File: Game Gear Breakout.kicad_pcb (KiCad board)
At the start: 2 copper layers, 59.1 x 73 mm, 11 parts, among them J1 GG Edge Connector, J2 Logic Analyzer, J3 ROM Chip

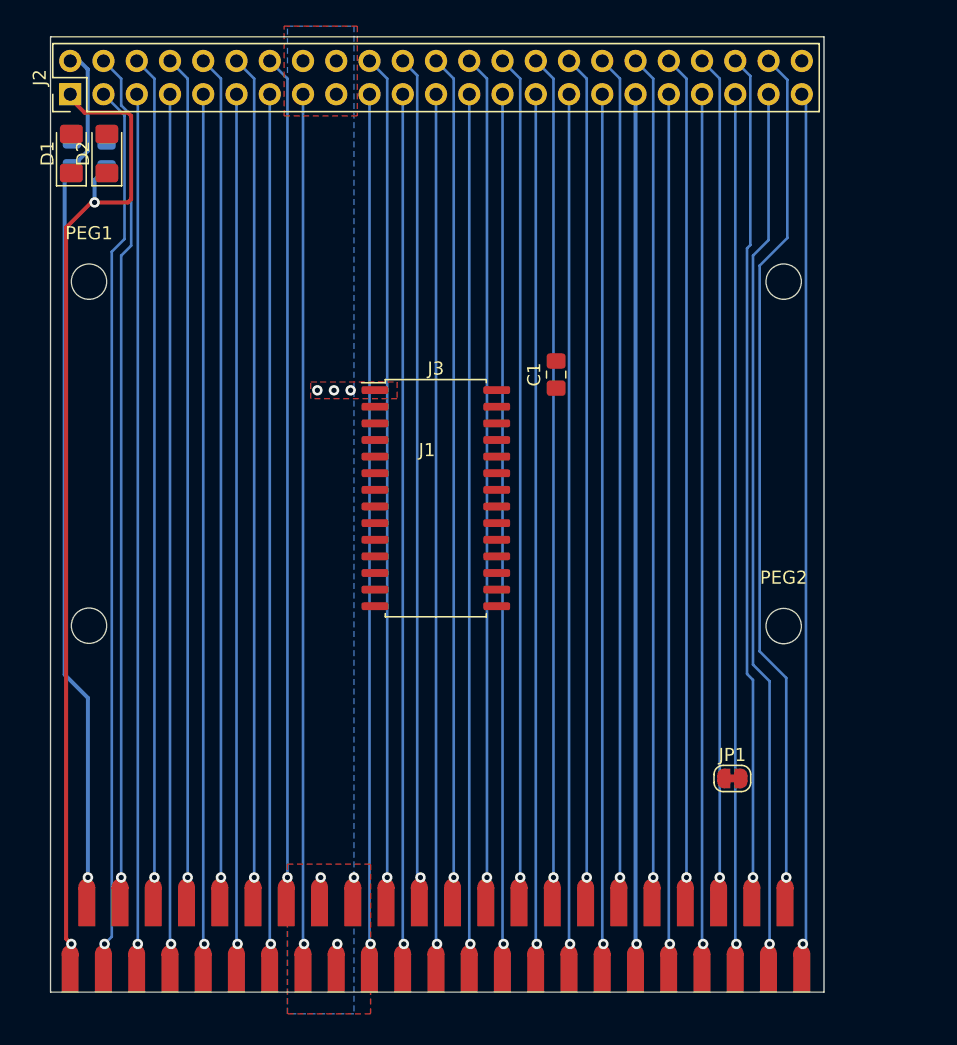
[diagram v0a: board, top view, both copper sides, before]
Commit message: rev1 layout done?
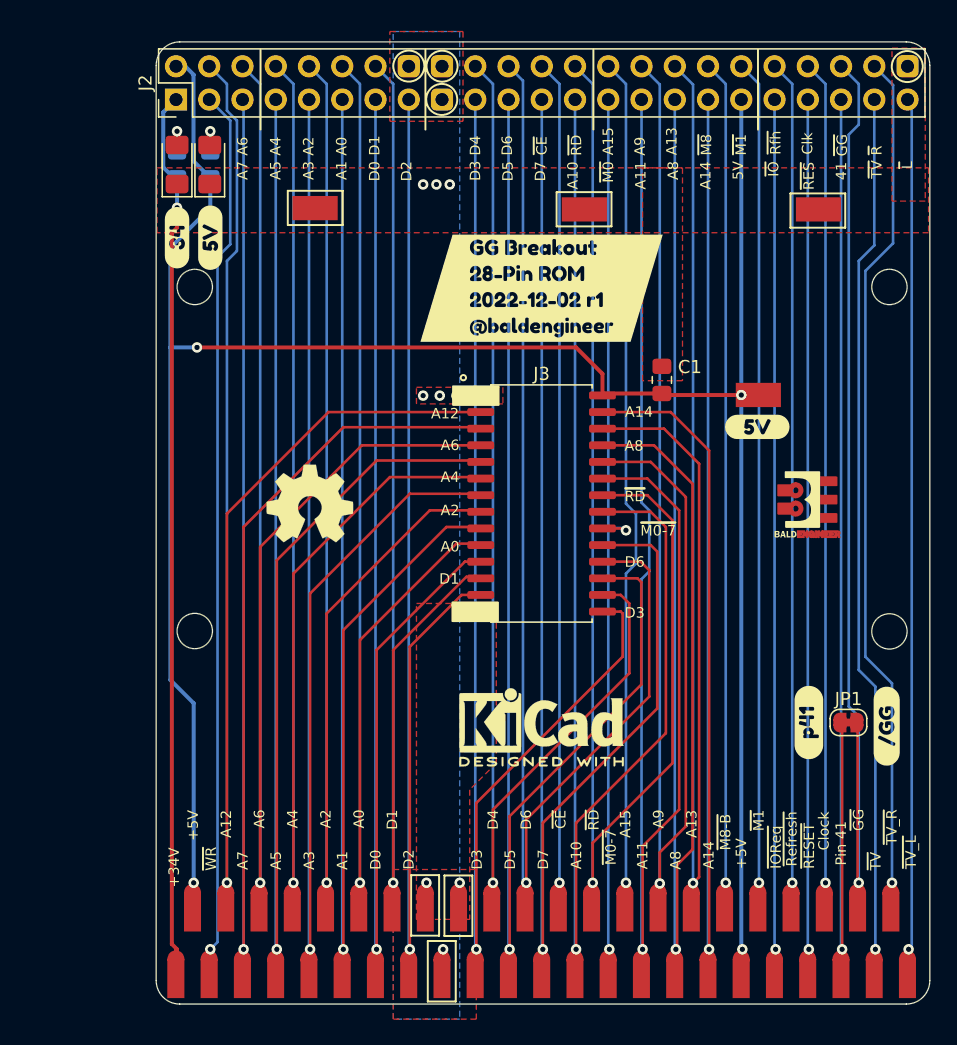
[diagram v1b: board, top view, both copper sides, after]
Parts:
- added REF**: OSHW-Symbol_6.7x6mm_SilkScreen, Symbol:OSHW-Symbol_6.7x6mm_SilkScreen, F.Cu at (145.0, 95.4)
- added REF**: KiCad-Logo2_5mm_SilkScreen, Symbol:KiCad-Logo2_5mm_SilkScreen, F.Cu at (162.7, 112.5)
- added TP1: TestPoint, My Libraries:Harwin-S1751-46-Test-Point, F.Cu at (165.9, 72.9)
- added TP2: TestPoint, My Libraries:Harwin-S1751-46-Test-Point, F.Cu at (183.8, 72.9)
- added TP3: TestPoint, My Libraries:Harwin-S1751-46-Test-Point, F.Cu at (145.4, 72.8)
- added TP4: TestPoint, My Libraries:Harwin-S1751-46-Test-Point, F.Cu at (179.2, 87.1)
- added kibuzzard-638A45B3: G***, kibuzzard-638A45B3, F.Cu at (137.4, 75.1)
- added kibuzzard-638A45B3: G***, kibuzzard-638A45B3, F.Cu at (179.1, 89.5)
- added kibuzzard-638A45BD: G***, kibuzzard-638A45BD, F.Cu at (134.8, 75.1)
- added kibuzzard-638A4743: G***, kibuzzard-638A4743, F.Cu at (189.0, 112.4)
- added kibuzzard-638A474E: G***, kibuzzard-638A474E, F.Cu at (183.1, 112.1)
- added kibuzzard-638A50E1: G***, kibuzzard-638A50E1, F.Cu at (162.7, 78.9)
- added svg2mod: G***, My Libraries:BE5v2, F.Cu at (180.5, 93.0)
- moved D1 10.6 mm to (137.3, 69.5)
- moved R1 10.6 mm to (137.4, 69.5)
- moved JP1 9.84 mm to (186.1, 112.1)
- moved C1 8.09 mm to (171.9, 85.9)
- moved J1 8.09 mm to (162.6, 103.2)
- moved J3 8.09 mm to (162.7, 95.4)
- moved PEG1 8.09 mm to (136.2, 78.8)
- moved PEG2 8.09 mm to (189.2, 105.2)
- moved J2 8.09 mm to (134.7, 64.5)
- moved R2 5.44 mm to (134.8, 69.5)
- moved D2 5.43 mm to (134.8, 69.5)
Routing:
- net /A7: track 67.2 -> 120.5 mm
- net /A12: track 65.8 -> 116.6 mm
- net /A5: track 67.2 -> 115.5 mm
- net /A14: track 67.2 -> 114.7 mm
- net +5V: track 134.3 -> 181.2 mm, vias 2 -> 4
- net /A6: track 65.2 -> 110.9 mm
- net /A8: track 67.2 -> 111.4 mm
- net /A3: track 67.2 -> 110.5 mm
- net /A11: track 67.2 -> 109.2 mm
- net /A4: track 65.2 -> 106.1 mm
- net /A13: track 65.2 -> 105.9 mm
- net /A10: track 67.2 -> 107.6 mm
- net /D7: track 67.2 -> 105.5 mm
- net /A1: track 67.2 -> 105.2 mm
- net /A9: track 65.2 -> 103.0 mm
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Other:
- board size 59.1 x 73 mm -> 59.1 x 73.5 mm
- board text added: "+34V"
- board text added: "+5V"
- board text added: "41"
- board text added: "5V"
- board text added: "A0"
- board text added: "A1"
- board text added: "A10"
- board text added: "A11"
- board text added: "A12"
- board text added: "A13"
- board text added: "A14"
- board text added: "A15"
- board text added: "A2"
- board text added: "A3"
- board text added: "A4"
- board text added: "A5"
- board text added: "A6"
- board text added: "A7"
- board text added: "A8"
- board text added: "A9"
- board text added: "Clk"
- board text added: "Clock"
- board text added: "D0"
- board text added: "D1"
- board text added: "D2"
- board text added: "D3"
- board text added: "D4"
- board text added: "D5"
- board text added: "D6"
- board text added: "D7"
- board text added: "Pin 41"
- board text added: "~{CE}"
- board text added: "~{GG}"
- board text added: "~{IOReq}"
- board text added: "~{IO}"
- board text added: "~{L}"
- board text added: "~{M0-7}"
- board text added: "~{M0}"
- board text added: "~{M1}"
- board text added: "~{M8-B}"
- board text added: "~{M8}"
- board text added: "~{RD}"
- board text added: "~{RESET}"
- board text added: "~{RES}"
- board text added: "~{Refresh}"
- board text added: "~{Rfh}"
- board text added: "~{R}"
- board text added: "~{TV_L}"
- board text added: "~{TV_R}"
- board text added: "~{TV}"
- board text added: "~{WR}"
